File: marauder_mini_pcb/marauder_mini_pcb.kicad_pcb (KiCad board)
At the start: 2 copper layers, 30 x 20 mm, 8 parts, among them J1 Conn_01x10, SW1 SW_SPDT, U1 ESP32-WROOM-32

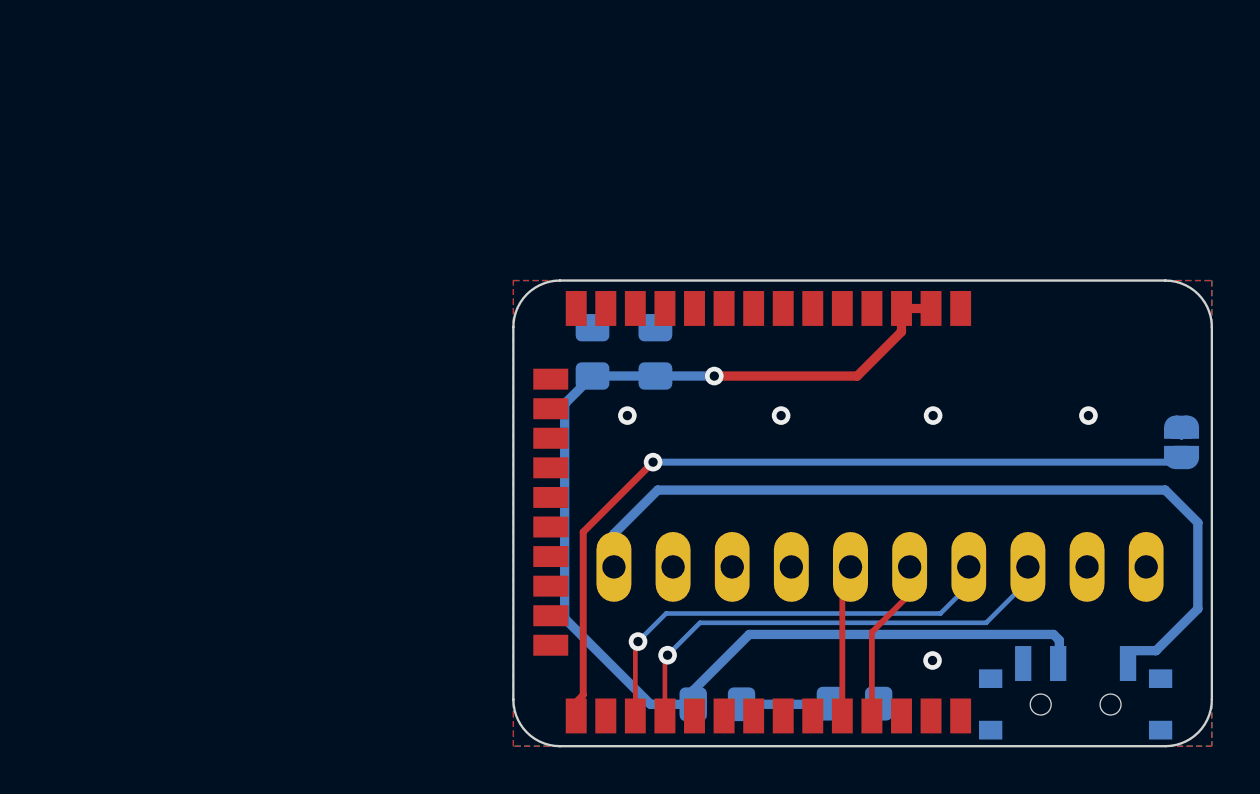
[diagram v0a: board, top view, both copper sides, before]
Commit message: Aggiornato circuito
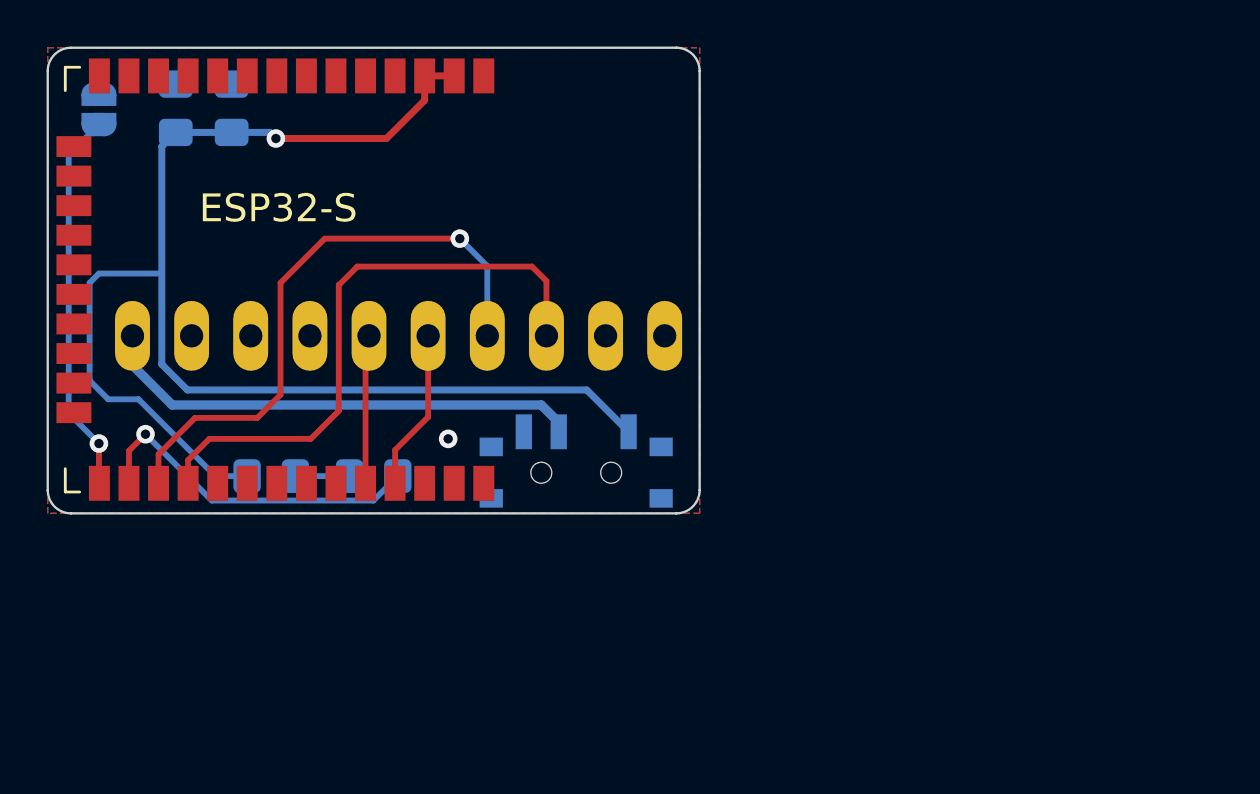
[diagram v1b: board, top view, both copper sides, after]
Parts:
- removed D1: LED, Capacitor_SMD:C_0805_2012Metric_Pad1.18x1.45mm_HandSolder
- removed PROG: SolderJumper_2_Open, Jumper:SolderJumper-2_P1.3mm_Open_RoundedPad1.0x1.5mm
- added JP1: SolderJumper_2_Open, Jumper:SolderJumper-2_P1.3mm_Open_RoundedPad1.0x1.5mm, B.Cu at (42.2, 42.6)
- added LED/IO04: LED, Capacitor_SMD:C_0805_2012Metric_Pad1.18x1.45mm_HandSolder, B.Cu at (54.0, 58.4)
- J1: footprint Connector_PinHeader_2.54mm:PinHeader_1x10_P2.54mm_Vertical -> Library:PinHeader_1x10_P2.54mm_Vertical_largo
- moved SW1 23.6 mm to (62.7, 57.9)
- moved C1 23.1 mm to (45.5, 42.6)
- moved J1 22.9 mm to (66.5, 52.4)
- moved U1 22.8 mm to (50.5, 50.0)
- moved R1 21.5 mm to (49.6, 58.4)
- moved C2 18.7 mm to (47.9, 42.6)
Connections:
- C1 pad 1: Net-(SW1-B) -> Net-(SW1-A)
- C2 pad 1: Net-(SW1-B) -> Net-(SW1-A)
- J1 pad 8: unconnected-(J1-Pin_8-Pad8) -> GND
- R1 pad 2: Net-(SW1-B) -> Net-(SW1-A)
- SW1 pad 1: Net-(J1-Pin_10) -> Net-(SW1-A)
- SW1 pad 2: Net-(SW1-B) -> Net-(J1-Pin_10)
- U1 pad 2: Net-(SW1-B) -> Net-(SW1-A)
- U1 pad 26: unconnected-(U1-IO4-Pad26) -> Net-(D1-K)
- U1 pad 3: Net-(SW1-B) -> Net-(SW1-A)
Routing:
- net Net-(SW1-A): track 0.00 -> 61.2 mm, vias 0 -> 1
- net Net-(SW1-B): track 52.5 -> 0.00 mm, vias 1 -> 0
- net Net-(JP1-A): track 35.0 -> 16.5 mm
- net Net-(D1-K): track 0.00 -> 14.9 mm, vias 0 -> 1
- net Net-(J1-Pin_10): track 35.7 -> 22.0 mm
- net Net-(J1-Pin_4): track 19.2 -> 25.5 mm
- net Net-(J1-Pin_3): track 20.1 -> 25.6 mm, vias 1 -> 0
- net Net-(D1-A): track 3.83 -> 2.32 mm
- net GND: track 0.35 -> 0.00 mm, vias 5 -> 1
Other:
- board size 30 x 20 mm -> 28 x 20 mm
- board text added: "ESP32-S"
- board text added: "Prog"
- board text removed: "OFF"
- board text removed: "ON"
- board text removed: "PROG"
